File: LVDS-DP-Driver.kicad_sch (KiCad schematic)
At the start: 15 parts

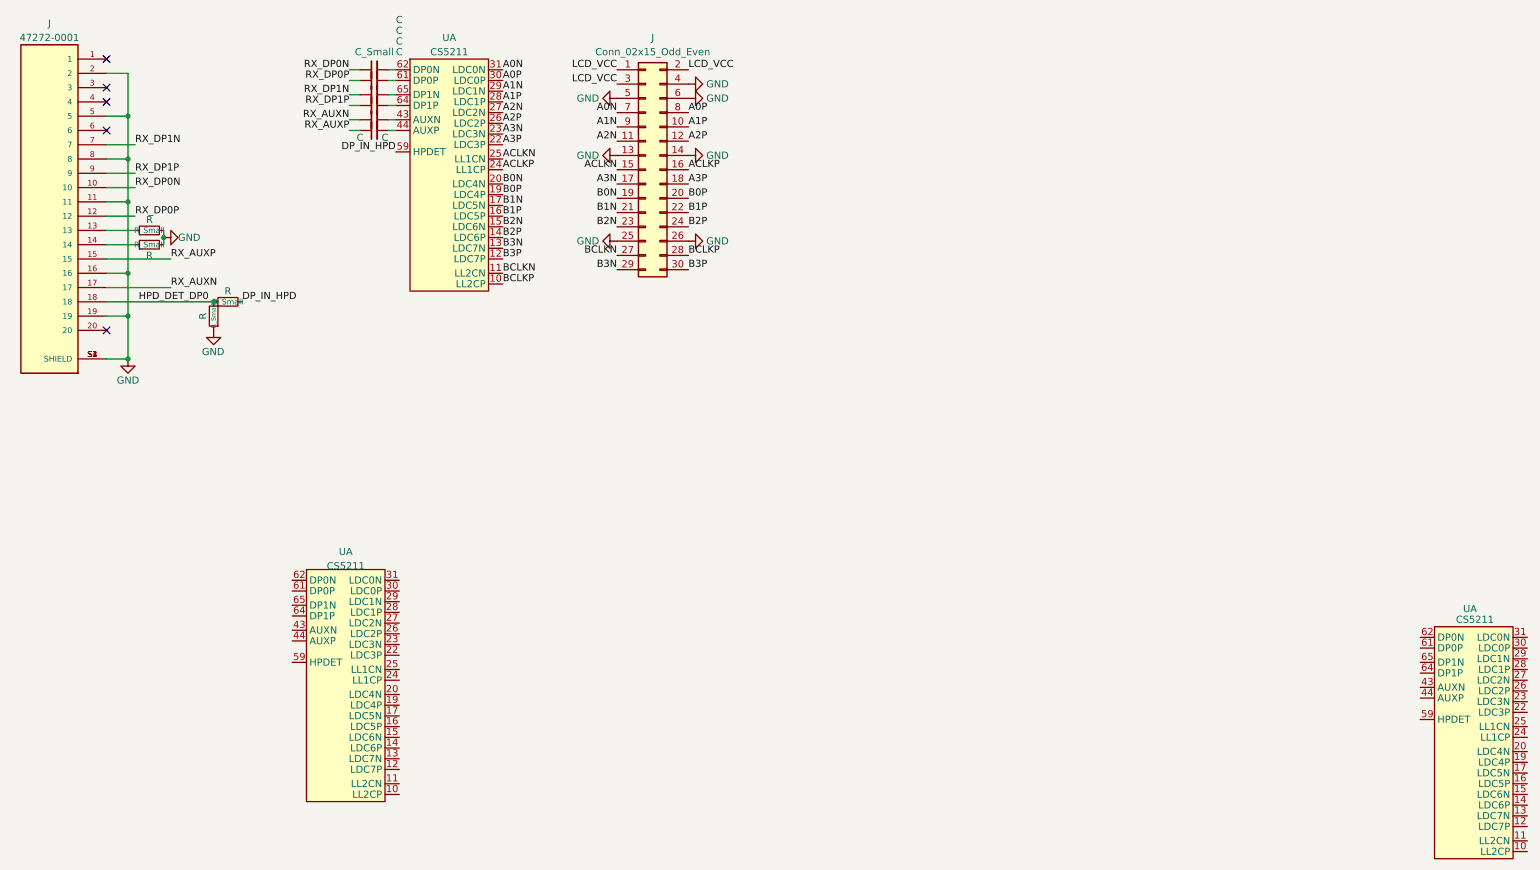
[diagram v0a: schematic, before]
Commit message: Power Management
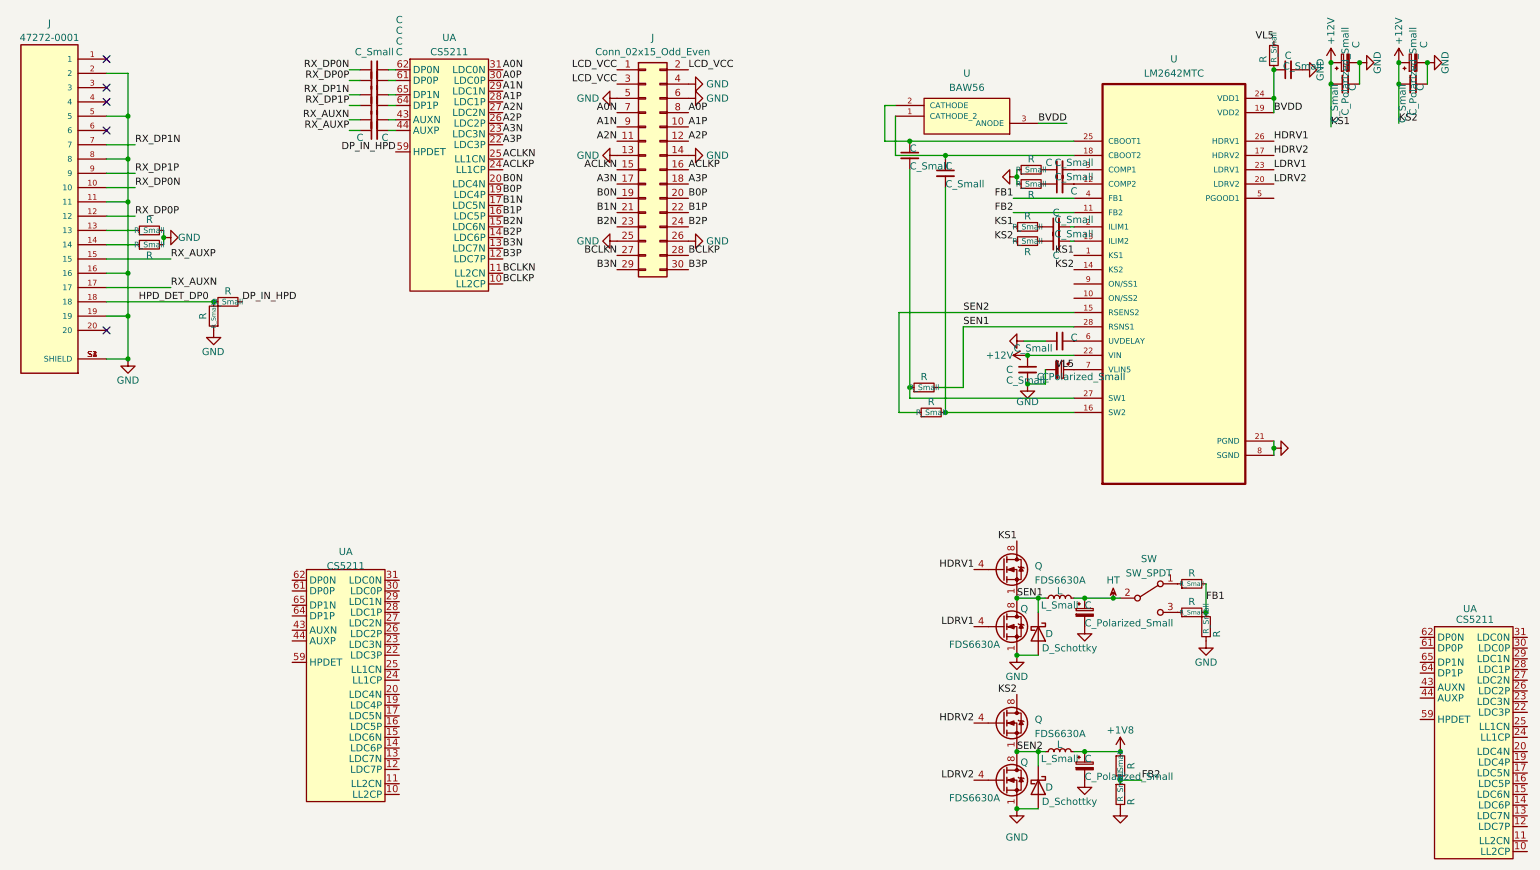
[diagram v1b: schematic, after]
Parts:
- added C (x5): C_Polarized_Small, symbol Device:C_Polarized_Small
- added C (x11): C_Small, symbol Device:C_Small
- added D (x2): D_Schottky, symbol Device:D_Schottky
- added L (x2): L_Small, symbol Device:L_Small
- added Q (x4): FDS6630A, Package_SO:SOIC-8_3.9x4.9mm_P1.27mm, symbol Transistor_FET:FDS6630A
- added R (x12): R_Small, symbol Device:R_Small
- added SW: SW_SPDT, symbol Switch:SW_SPDT
- added U: BAW56, SOT95P240X110-3N, symbol BAW56:BAW56
- added U: LM2642MTC, SOP65P640X120-28N, symbol LM2642MTC:LM2642MTC
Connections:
- net GND: now also C.1, C.1, C.1, C.2, C.2, C.2, C.2, C.2, C.2, C.2, D.2 (A), D.2 (A), Q.1 (S), Q.1 (S), Q.2 (S), Q.2 (S), Q.3 (S), Q.3 (S), R.1, R.1, R.2, R.2, U.21 (PGND), U.8 (SGND)
- new net: C.2, R.1, U.27 (SW1)
- new net: C.1, U.2 (CATHODE), U.25 (CBOOT1)
- new net: R.1, SW.1 (A)
- new net: R.1, SW.3 (C)
- new net: C.1, U.1 (CATHODE_2), U.18 (CBOOT2)
- new net: C.1, R.2 (x4)
- new net: C.2, U.13 (ILIM2)
- new net: C.2, R.2, U.16 (SW2)
- new net: C.2, U.3 (COMP1)
- new net: C.2, U.6 (UVDELAY)
- new net: C.2, U.12 (COMP2)
- new net: C.2, U.2 (ILIM1)
- new net +12V: C.1, C.1, C.1, C.2, C.2, Q.5 (D), Q.5 (D), Q.6 (D), Q.6 (D), Q.7 (D), Q.7 (D), Q.8 (D), Q.8 (D), R.1, R.1, U.1 (KS1), U.14 (KS2), U.22 (VIN)
- new net +1V8: C.1, L.2, R.1
- new net BVDD: C.1, R.2, U.19 (VDD2), U.24 (VDD1), U.3 (ANODE)
- new net FB1: R.1, R.2, R.2, U.4 (FB1)
- new net FB2: R.1, R.2, U.11 (FB2)
- new net HDRV1: Q.4 (G), U.26 (HDRV1)
- new net HDRV2: Q.4 (G), U.17 (HDRV2)
- new net HT: C.1, L.2, SW.2 (B)
- new net LDRV1: Q.4 (G), U.23 (LDRV1)
- new net LDRV2: Q.4 (G), U.20 (LDRV2)
- new net SEN1: D.1 (K), L.1, Q.1 (S), Q.2 (S), Q.3 (S), Q.5 (D), Q.6 (D), Q.7 (D), Q.8 (D), R.2, U.28 (RSNS1)
- new net SEN2: D.1 (K), L.1, Q.1 (S), Q.2 (S), Q.3 (S), Q.5 (D), Q.6 (D), Q.7 (D), Q.8 (D), R.1, U.15 (RSENS2)
- new net VL5: C.1, R.1, U.7 (VLIN5)
